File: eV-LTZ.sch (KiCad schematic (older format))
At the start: 28 parts, among them M1 SGP2, M2 SGP2, M3 SGP2, P1 CONN_01X04, P2 CONN_01X02, Q1 Q_NPN_EBC, U1 LT1013

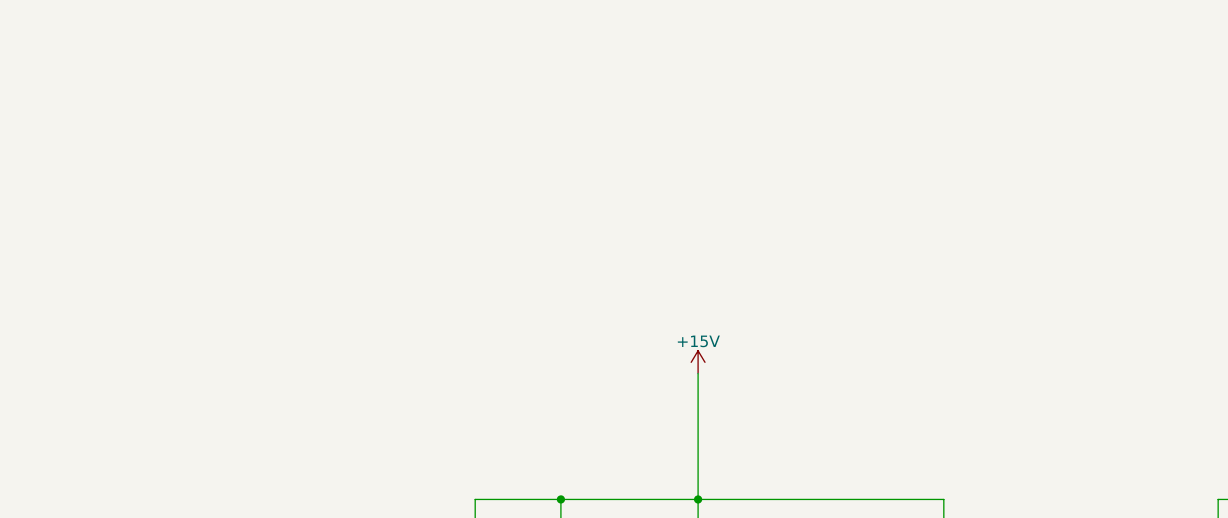
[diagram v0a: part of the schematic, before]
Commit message: TiN comments
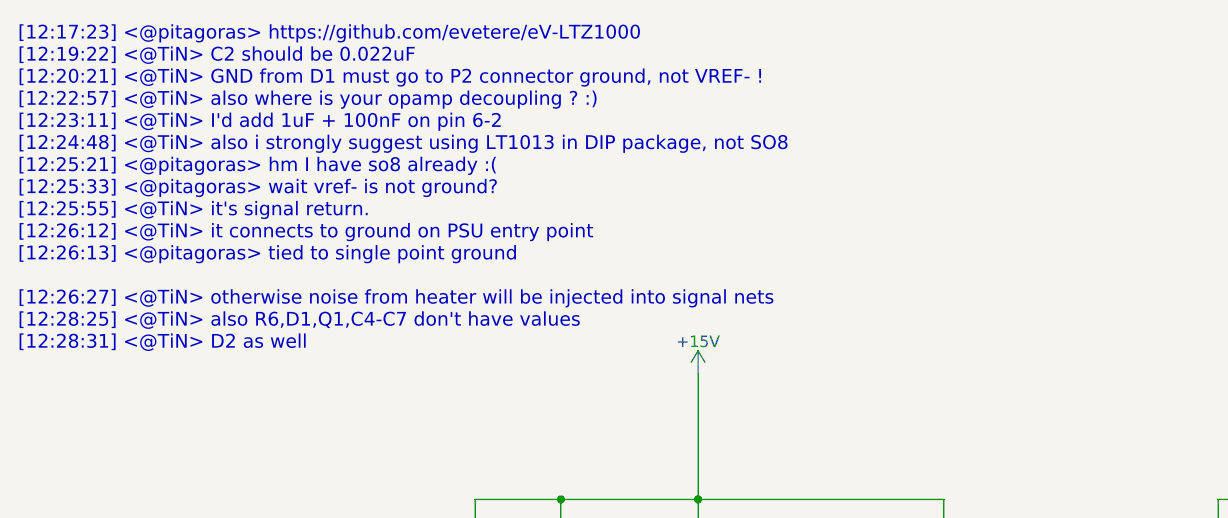
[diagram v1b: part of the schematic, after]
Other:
- note added: "[12:17:23] <@pitagoras> https://github.com/evetere/eV-LTZ1000\n[12:19:22] <@TiN> C2 should be 0.022uF\n[12:20:21] <@TiN> GND from D1 must go to P2 connector ground, not VREF- !\n[12:22:57] <@TiN> also where is your opamp decoupling ? :)\n[12:23:11] <@TiN> I'd add 1uF + 100nF on pin 6-2\n[12:24:48] <@TiN> also i strongly suggest using LT1013 in DIP package, not SO8\n[12:25:21] <@pitagoras> hm I ha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"
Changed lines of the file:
@@
 LIBS:valves
 LIBS:eV-LTZ1000
-LIBS:pi-LTZ-cache
+LIBS:eV-LTZ-cache
 EELAYER 25 0
 EELAYER END
@@
 Wire Wire Line
 	6300 3000 6300 2875
+Text Notes 1050 1900 0    60   ~ 0
+[12:17:23] <@pitagoras> https://github.com/evetere/eV-LTZ1000\n[12:19:22] <@TiN> C2 should be 0.022uF\n[12:20:21] <@TiN> GND from D1 must go to P2 connector ground, not VREF- !\n[12:22:57] <@TiN> also where is your opamp decoupling ? :)\n[12:23:11] <@TiN> I'd add 1uF + 100nF on pin 6-2\n[12:24:48] <@TiN> also i strongly suggest using LT1013 in DIP package, not SO8\n[12:25:21] <@pitagoras> hm I have so8 already :(\n[12:25:33] <@pitagoras> wait vref- is not ground?\n[12:25:55] <@TiN> it's signal return.\n[12:26:12] <@TiN> it connects to ground on PSU entry point\n[12:26:13] <@pitagoras> tied to single point ground \n\n[12:26:27] <@TiN> otherwise noise from heater will be injected into signal nets\n[12:28:25] <@TiN> also R6,D1,Q1,C4-C7 don't have values\n[12:28:31] <@TiN> D2 as well\n\n
 $EndSCHEMATC

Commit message: fix TiN comments
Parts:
- removed C5: C, symbol C
- added C? (x2): 1u, symbol CP
- C2: value 0.002uF -> 0.022uF
- C4, C6: value C -> 100n
- C7: value C -> 0.022uF
- D1, D2: value D -> 1N4148
- P1: value CONN_01X04 -> REF
- P2: value CONN_01X02 -> PWR
- Q1: value Q_NPN_EBC -> 2N3904
- R6: value R -> 1k
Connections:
- wire segments 82 -> 85
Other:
- note removed: "[12:17:23] <@pitagoras> https://github.com/evetere/eV-LTZ1000\n[12:19:22] <@TiN> C2 should be 0.022uF\n[12:20:21] <@TiN> GND from D1 must go to P2 connector ground, not VREF- !\n[12:22:57] <@TiN> also where is your opamp decoupling ? :)\n[12:23:11] <@TiN> I'd add 1uF + 100nF on pin 6-2\n[12:24:48] <@TiN> also i strongly suggest using LT1013 in DIP package, not SO8\n[12:25:21] <@pitagoras> hm I ha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"
- moved on the sheet: C1, C6, C7, M3, R7
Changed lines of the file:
@@
 LIBS:valves
 LIBS:eV-LTZ1000
-LIBS:eV-LTZ-cache
 EELAYER 25 0
 EELAYER END
@@
 P 4500 3250
 F 0 "R6" V 4580 3250 50  0000 C CNN
-F 1 "R" V 4500 3250 50  0000 C CNN
+F 1 "1k" V 4500 3250 50  0000 C CNN
 F 2 "" V 4430 3250 50  0001 C CNN
 F 3 "" H 4500 3250 50  0000 C CNN
@@
 P 4525 4925
 F 0 "D1" H 4525 5025 50  0000 C CNN
-F 1 "D" H 4525 4825 50  0000 C CNN
+F 1 "1N4148" H 4525 4825 50  0000 C CNN
 F 2 "" H 4525 4925 50  0001 C CNN
 F 3 "" H 4525 4925 50  0000 C CNN
@@
 L C C1
 U 1 1 591A85DA
-P 5450 3900
-F 0 "C1" H 5475 4000 50  0000 L CNN
-F 1 ".1uF" H 5475 3800 50  0000 L CNN
-F 2 "" H 5488 3750 50  0001 C CNN
-F 3 "" H 5450 3900 50  0000 C CNN
-	1    5450 3900
+P 5600 3900
+F 0 "C1" H 5625 4000 50  0000 L CNN
+F 1 ".1uF" H 5625 3800 50  0000 L CNN
+F 2 "" H 5638 3750 50  0001 C CNN
+F 3 "" H 5600 3900 50  0000 C CNN
+	1    5600 3900
 	1    0    0    -1
 $EndComp
@@
 L R R7
 U 1 1 591A8697
-P 5450 3550
-F 0 "R7" V 5530 3550 50  0000 C CNN
-F 1 "1M" V 5450 3550 50  0000 C CNN
-F 2 "" V 5380 3550 50  0001 C CNN
-F 3 "" H 5450 3550 50  0000 C CNN
-	1    5450 3550
+P 5600 3550
+F 0 "R7" V 5680 3550 50  0000 C CNN
+F 1 "1M" V 5600 3550 50  0000 C CNN
+F 2 "" V 5530 3550 50  0001 C CNN
+F 3 "" H 5600 3550 50  0000 C CNN
+	1    5600 3550
 	1    0    0    -1
 $EndComp
@@
 P 9400 2675
 F 0 "D2" H 9400 2775 50  0000 C CNN
-F 1 "D" H 9400 2575 50  0000 C CNN
+F 1 "1N4148" H 9400 2575 50  0000 C CNN
 F 2 "" H 9400 2675 50  0001 C CNN
 F 3 "" H 9400 2675 50  0000 C CNN
@@
 P 8300 4025
 F 0 "C2" H 8325 4125 50  0000 L CNN
-F 1 "0.002uF" H 8325 3925 50  0000 L CNN
+F 1 "0.022uF" H 8325 3925 50  0000 L CNN
 F 2 "" H 8338 3875 50  0001 C CNN
 F 3 "" H 8300 4025 50  0000 C CNN
@@
 L GND #PWR2
 U 1 1 591A9570
-P 5600 5150
-F 0 "#PWR2" H 5600 4900 50  0001 C CNN
-F 1 "GND" H 5600 5000 50  0000 C CNN
-F 2 "" H 5600 5150 50  0000 C CNN
-F 3 "" H 5600 5150 50  0000 C CNN
-	1    5600 5150
+P 3425 5450
+F 0 "#PWR2" H 3425 5200 50  0001 C CNN
+F 1 "GND" H 3425 5300 50  0000 C CNN
+F 2 "" H 3425 5450 50  0000 C CNN
+F 3 "" H 3425 5450 50  0000 C CNN
+	1    3425 5450
 	1    0    0    -1
 $EndComp
@@
 P 10150 3550
 F 0 "P1" H 10150 3800 50  0000 C CNN
-F 1 "CONN_01X04" V 10250 3550 50  0000 C CNN
+F 1 "REF" V 10250 3550 50  0000 C CNN
 F 2 "" H 10150 3550 50  0001 C CNN
 F 3 "" H 10150 3550 50  0000 C CNN
@@
 P 4125 3250
 F 0 "Q1" H 4325 3300 50  0000 L CNN
-F 1 "Q_NPN_EBC" H 4325 3200 50  0000 L CNN
+F 1 "2N3904" H 4325 3200 50  0000 L CNN
 F 2 "" H 4325 3350 50  0000 C CNN
 F 3 "" H 4125 3250 50  0000 C CNN
@@
 L SGP2 M3
 U 1 1 59BA1924
-P 9650 4100
-F 0 "M3" H 9425 4100 60  0000 C CNN
-F 1 "SGP2" H 9425 3875 60  0001 C CNN
-F 2 "" H 9175 4225 60  0001 C CNN
-F 3 "" H 9175 4225 60  0001 C CNN
-	1    9650 4100
-	1    0    0    -1
+P 3625 5225
+F 0 "M3" H 3400 5225 60  0000 C CNN
+F 1 "SGP2" H 3400 5000 60  0001 C CNN
+F 2 "" H 3150 5350 60  0001 C CNN
+F 3 "" H 3150 5350 60  0001 C CNN
+	1    3625 5225
+	-1   0    0    1
 $EndComp
 $Comp
@@
 Text Label 8725 3825 0    60   ~ 0
 SENSE-
-Text Label 9800 4100 0    60   ~ 0
+Text Label 9800 4000 0    60   ~ 0
 VREF-
 $Comp
@@
 P 2625 3275
 F 0 "P2" H 2625 3425 50  0000 C CNN
-F 1 "CONN_01X02" V 2725 3275 50  0000 C CNN
+F 1 "PWR" V 2725 3275 50  0000 C CNN
 F 2 "" H 2625 3275 50  0000 C CNN
 F 3 "" H 2625 3275 50  0000 C CNN
@@
 L C C7
 U 1 1 59BC10DD
-P 4825 2800
-F 0 "C7" H 4850 2900 50  0000 L CNN
-F 1 "C" H 4850 2700 50  0000 L CNN
-F 2 "" H 4863 2650 50  0000 C CNN
-F 3 "" H 4825 2800 50  0000 C CNN
-	1    4825 2800
+P 4825 3575
+F 0 "C7" H 4850 3675 50  0000 L CNN
+F 1 "0.022uF" H 4850 3475 50  0000 L CNN
+F 2 "" H 4863 3425 50  0000 C CNN
+F 3 "" H 4825 3575 50  0000 C CNN
+	1    4825 3575
 	0    1    1    0
-$EndComp
-$Comp
-L C C5
-U 1 1 59BC16B9
-P 3425 3750
-F 0 "C5" H 3450 3850 50  0000 L CNN
-F 1 "C" H 3450 3650 50  0000 L CNN
-F 2 "" H 3463 3600 50  0000 C CNN
-F 3 "" H 3425 3750 50  0000 C CNN
-	1    3425 3750
-	1    0    0    -1
 $EndComp
 $Comp
 L C C6
 U 1 1 59BC172F
-P 3650 3750
-F 0 "C6" H 3675 3850 50  0000 L CNN
-F 1 "C" H 3675 3650 50  0000 L CNN
-F 2 "" H 3688 3600 50  0000 C CNN
-F 3 "" H 3650 3750 50  0000 C CNN
-	1    3650 3750
-	1    0    0    -1
-$EndComp
-$Comp
-L C C4
-U 1 1 59BC1B82
-P 3200 3750
-F 0 "C4" H 3225 3850 50  0000 L CNN
-F 1 "C" H 3225 3650 50  0000 L CNN
-F 2 "" H 3238 3600 50  0000 C CNN
-F 3 "" H 3200 3750 50  0000 C CNN
-	1    3200 3750
+P 5400 3850
+F 0 "C6" H 5425 3950 50  0000 L CNN
+F 1 "100n" H 5425 3750 50  0000 L CNN
+F 2 "" H 5438 3700 50  0000 C CNN
+F 3 "" H 5400 3850 50  0000 C CNN
+	1    5400 3850
 	1    0    0    -1
 $EndComp
@@
 	4025 3450 4025 4125
 Wire Wire Line
-	5450 4050 5450 4100
+	5600 4050 5600 4100
 Wire Wire Line
 	4025 4100 5900 4100
@@
 	5300 3350 5775 3350
 Wire Wire Line
-	5450 3400 5450 3350
-Connection ~ 5450 3350
-Wire Wire Line
-	5450 3700 5450 3750
+	5600 3400 5600 3350
+Connection ~ 5600 3350
+Wire Wire Line
+	5600 3700 5600 3750
 Wire Wire Line
 	4375 4925 4025 4925
 Wire Wire Line
 	4025 4925 4025 4900
-Wire Wire Line
-	4675 4925 9425 4925
 Connection ~ 5100 4925
 Wire Wire Line
 	6800 3550 6800 3650
-Connection ~ 5450 4100
+Connection ~ 5600 4100
 Wire Wire Line
 	5725 2975 5725 4150
@@
 	5100 2450 5100 2950
 Wire Wire Line
-	3050 2450 5100 2450
+	3050 2450 5400 2450
 Connection ~ 4025 2450
 Wire Wire Line
-	5725 4750 9100 4750
-Wire Wire Line
-	5100 5225 5100 3550
+	5325 4750 9100 4750
 Connection ~ 6300 4750
 Connection ~ 7200 4750
@@
 	6800 3650 7800 3650
 Wire Wire Line
-	9425 4925 9425 4200
-Wire Wire Line
-	9425 4200 9550 4200
-Wire Wire Line
 	9100 4750 9100 4000
 Wire Wire Line
-	9100 4000 9550 4000
+	9100 4000 9800 4000
 Wire Wire Line
 	9600 3600 9950 3600
 Wire Wire Line
-	9650 4100 9800 4100
-Wire Wire Line
-	9800 4100 9800 3700
-Wire Wire Line
 	9800 3700 9950 3700
 Wire Wire Line
@@
 	9600 3825 9600 3600
 Wire Wire Line
-	5600 5150 5600 4925
-Connection ~ 5600 4925
+	3425 3900 3425 5450
+Connection ~ 3425 5225
 Wire Wire Line
 	2825 3225 3050 3225
@@
 	3050 3325 3050 5225
 Wire Wire Line
-	3050 5225 5100 5225
-Wire Wire Line
-	4975 2800 5325 2800
-Wire Wire Line
-	5325 2800 5325 3350
-Connection ~ 5325 3350
+	4975 3575 5300 3575
+Connection ~ 5300 3350
 Connection ~ 4675 3250
-Wire Wire Line
-	4675 3250 4675 2800
 Wire Wire Line
 	3425 2450 3425 3600
 Connection ~ 3425 2450
-Wire Wire Line
-	3200 3900 3650 3900
 Connection ~ 3425 3900
 Wire Wire Line
 	3200 3600 3200 3500
-Wire Wire Line
-	3200 3500 3650 3500
 Connection ~ 3425 3500
 Wire Wire Line
-	3650 3500 3650 3600
-Wire Wire Line
-	3425 3900 3425 5225
-Connection ~ 3425 5225
-Wire Wire Line
 	6300 3000 6300 2875
-Text Notes 1050 1900 0    60   ~ 0
-[12:17:23] <@pitagoras> https://github.com/evetere/eV-LTZ1000\n[12:19:22] <@TiN> C2 should be 0.022uF\n[12:20:21] <@TiN> GND from D1 must go to P2 connector ground, not VREF- !\n[12:22:57] <@TiN> also where is your opamp decoupling ? :)\n[12:23:11] <@TiN> I'd add 1uF + 100nF on pin 6-2\n[12:24:48] <@TiN> also i strongly suggest using LT1013 in DIP package, not SO8\n[12:25:21] <@pitagoras> hm I have so8 already :(\n[12:25:33] <@pitagoras> wait vref- is not ground?\n[12:25:55] <@TiN> it's signal return.\n[12:26:12] <@TiN> it connects to ground on PSU entry point\n[12:26:13] <@pitagoras> tied to single point ground \n\n[12:26:27] <@TiN> otherwise noise from heater will be injected into signal nets\n[12:28:25] <@TiN> also R6,D1,Q1,C4-C7 don't have values\n[12:28:31] <@TiN> D2 as well\n\n
+Wire Wire Line
+	5300 3575 5300 3350
+Wire Wire Line
+	4675 3575 4675 3250
+$Comp
+L CP C?
+U 1 1 59CD714F
+P 5200 3850
+F 0 "C?" H 5225 3950 50  0000 L CNN
+F 1 "1u" H 5225 3750 50  0000 L CNN
+F 2 "" H 5238 3700 50  0000 C CNN
+F 3 "" H 5200 3850 50  0000 C CNN
+	1    5200 3850
+	1    0    0    -1
+$EndComp
+Wire Wire Line
+	5100 4050 5400 4050
+Wire Wire Line
+	5400 4050 5400 4000
+Connection ~ 5100 4050
+Wire Wire Line
+	5200 4000 5200 4050
+Connection ~ 5200 4050
+Wire Wire Line
+	5200 3700 5400 3700
+Wire Wire Line
+	5400 3700 5400 2450
+Connection ~ 5100 2450
+$Comp
+L C C4
+U 1 1 59BC1B82
+P 3200 3750
+F 0 "C4" H 3225 3850 50  0000 L CNN
+F 1 "100n" H 3225 3650 50  0000 L CNN
+F 2 "" H 3238 3600 50  0000 C CNN
+F 3 "" H 3200 3750 50  0000 C CNN
+	1    3200 3750
+	1    0    0    -1
+$EndComp
+$Comp
+L CP C?
+U 1 1 59CD7798
+P 3425 3750
+F 0 "C?" H 3450 3850 50  0000 L CNN
+F 1 "1u" H 3450 3650 50  0000 L CNN
+F 2 "" H 3463 3600 50  0000 C CNN
+F 3 "" H 3425 3750 50  0000 C CNN
+	1    3425 3750
+	1    0    0    -1
+$EndComp
+Wire Wire Line
+	3200 3500 3425 3500
+Wire Wire Line
+	3200 3900 3425 3900
+Wire Wire Line
+	3050 5225 3625 5225
+Wire Wire Line
+	5100 4925 4675 4925
+Wire Wire Line
+	5100 5125 3725 5125
+Wire Wire Line
+	5325 5325 3725 5325
+Wire Wire Line
+	5325 4750 5325 5325
+Wire Wire Line
+	5100 3550 5100 5125
+Connection ~ 5725 4750
+Wire Wire Line
+	9800 4000 9800 3700
 $EndSCHEMATC

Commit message: guard ring
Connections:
- wire segments 85 -> 120
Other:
- note added: "guard ring"
- moved on the sheet: C1, C4, C6, C7, D1, M3, P2, Q1, R6, R7, U1A

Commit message: updates
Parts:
- removed C?: 1u, symbol CP
- removed M1, M2, M3: SGP2, symbol SGP2
- removed P1: REF, symbol CONN_01X04
- removed Q1: 2N3904, symbol Q_NPN_EBC
- removed R4.3: 0k, symbol R
- removed U1: LT1013, symbol LT1013
- added C10, C5: 1uF, Capacitors_THT:CP_Radial_Tantal_D5.0mm_P5.00mm, symbol CP
- added C9: .1uF, Capacitors_THT:C_Rect_L7.2mm_W2.5mm_P5.00mm_FKS2_FKP2_MKS2_MKP2, symbol C
- added D3, D6: 1N5819, Diodes_THT:D_DO-41_SOD81_P10.16mm_Horizontal, symbol D_Shockley
- added D4, D5, D7: D_TVS, Diodes_THT:D_DO-15_P10.16mm_Horizontal, symbol D_TVS
- added P1: VIN+, Connectors:1pin, symbol CONN_01X01
- added P3: VH-, Connectors:1pin, symbol CONN_01X01
- added P4: VH+, Connectors:1pin, symbol CONN_01X01
- added P5: SENSE-, Connectors:1pin, symbol CONN_01X01
- added P6: SENSE+, Connectors:1pin, symbol CONN_01X01
- added P7: VIN-, Connectors:1pin, symbol CONN_01X01
- added Q1: BD139, TO_SOT_Packages_THT:TO-126_Vertical, symbol BD139
- added R4: 100k, Resistors_THT:R_Axial_DIN0309_L9.0mm_D3.2mm_P12.70mm_Horizontal, symbol R
- added TH1: 10k, Varistors:RV_Disc_D7_W3.4_P5, symbol Thermistor_NTC
- added U1: LT1013N8, Housings_DIP:DIP-8_W7.62mm, symbol LT1013N8
- added W1: TEST_HEATER, Connectors:PINTST, symbol TEST_1P
- added W2: TEST_SENSE, Connectors:PINTST, symbol TEST_1P
- C1, C2, C7: footprint (none) -> Capacitors_THT:C_Rect_L7.2mm_W2.5mm_P5.00mm_FKS2_FKP2_MKS2_MKP2
- C3: value 0.1uF -> .1uF; footprint (none) -> Capacitors_THT:C_Rect_L7.2mm_W2.5mm_P5.00mm_FKS2_FKP2_MKS2_MKP2
- C4, C6: value 100n -> .1uF; footprint (none) -> Capacitors_THT:C_Rect_L7.2mm_W2.5mm_P5.00mm_FKS2_FKP2_MKS2_MKP2
- C8: renamed from C?; value 1u -> 1uF; footprint (none) -> Capacitors_THT:CP_Radial_Tantal_D5.0mm_P5.00mm
- D1, D2: footprint (none) -> Diodes_THT:D_A-405_P7.62mm_Horizontal
- P2: value PWR -> CONN_01X02; footprint (none) -> Connectors:bornier2
- R1, R2, R3, R4.1, R4.2, R5: footprint (none) -> Resistors_THT:R_Axial_DIN0614_L14.3mm_D5.7mm_P15.24mm_Horizontal
- R6, R7, R8, R9: footprint (none) -> Resistors_THT:R_Axial_DIN0309_L9.0mm_D3.2mm_P12.70mm_Horizontal
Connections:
- net labels added: HEAT, TSENSE, VH+, VH-, VIN+, VIN-
- net labels removed: +15V, VREF-
- wire segments 120 -> 97
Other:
- moved on the sheet: C1, C2, C3, C4, C6, C7, D1, D2, R1, R2, R3, R4.1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

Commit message: pcb
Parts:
- removed C8: 1uF, Capacitors_THT:CP_Radial_Tantal_D5.0mm_P5.00mm, symbol CP
- removed C9: .1uF, Capacitors_THT:C_Rect_L7.2mm_W2.5mm_P5.00mm_FKS2_FKP2_MKS2_MKP2, symbol C
- removed D4, D5, D7: D_TVS, Diodes_THT:D_DO-15_P10.16mm_Horizontal, symbol D_TVS
- C10, C5: value 1uF -> 47uF
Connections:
- wire segments 97 -> 89
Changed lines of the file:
@@
-$EndComp
-$Comp
-L CP C8
-U 1 1 59CD714F
-P 5175 2975
-F 0 "C8" H 5200 3075 50  0000 L CNN
-F 1 "1uF" H 5200 2875 50  0000 L CNN
-F 2 "Capacitors_THT:CP_Radial_Tantal_D5.0mm_P5.00mm" H 5213 2825 50  0001 C CNN
-F 3 "" H 5175 2975 50  0000 C CNN
-	1    5175 2975
-	1    0    0    -1
 $EndComp
 $Comp
@@
 	1    6300 925
 	1    0    0    -1
-$EndComp
-$Comp
-L D_TVS D5
-U 1 1 59EE5901
-P 1650 3125
-F 0 "D5" H 1650 3225 50  0000 C CNN
-F 1 "D_TVS" H 1650 3025 50  0000 C CNN
-F 2 "Diodes_THT:D_DO-15_P10.16mm_Horizontal" H 1650 3125 50  0001 C CNN
-F 3 "" H 1650 3125 50  0000 C CNN
-	1    1650 3125
-	0    1    1    0
 $EndComp
 $Comp
@@
 $EndComp
 $Comp
-L C C9
-U 1 1 59FDB55A
-P 3050 3275
-F 0 "C9" H 3075 3375 50  0000 L CNN
-F 1 ".1uF" H 3075 3175 50  0000 L CNN
-F 2 "Capacitors_THT:C_Rect_L7.2mm_W2.5mm_P5.00mm_FKS2_FKP2_MKS2_MKP2" H 3088 3125 50  0001 C CNN
-F 3 "" H 3050 3275 50  0000 C CNN
-	1    3050 3275
-	1    0    0    -1
-$EndComp
-$Comp
 L D_Shockley D6
 U 1 1 59FDD6C1
@@
 	1    0    0    -1
 $EndComp
-$Comp
-L D_TVS D4
-U 1 1 59FDF05E
-P 1900 3125
-F 0 "D4" H 1900 3225 50  0000 C CNN
-F 1 "D_TVS" H 1900 3025 50  0000 C CNN
-F 2 "Diodes_THT:D_DO-15_P10.16mm_Horizontal" H 1900 3125 50  0001 C CNN
-F 3 "" H 1900 3125 50  0000 C CNN
-	1    1900 3125
-	0    1    1    0
-$EndComp
 Wire Wire Line
 	6325 2475 6750 2475
@@
 Connection ~ 5075 3175
 Wire Wire Line
-	5175 3125 5175 3175
-Connection ~ 5175 3175
-Wire Wire Line
-	5375 2825 5175 2825
-Wire Wire Line
 	5375 1475 5375 2825
 Connection ~ 5075 1475
@@
 	1900 1675 1900 2975
 Connection ~ 1900 1675
-$Comp
-L D_TVS D7
-U 1 1 59FE08AF
-P 10100 2525
-F 0 "D7" H 10100 2625 50  0000 C CNN
-F 1 "D_TVS" H 10100 2425 50  0000 C CNN
-F 2 "Diodes_THT:D_DO-15_P10.16mm_Horizontal" H 10100 2525 50  0001 C CNN
-F 3 "" H 10100 2525 50  0000 C CNN
-	1    10100 2525
-	0    1    1    0
-$EndComp
-Wire Wire Line
-	10100 1925 10100 2375
 Connection ~ 10100 1925
-Wire Wire Line
-	10100 2675 10100 3075
 Connection ~ 10100 3075
 $Comp
@@
 	4000 4100 4000 4025
 Connection ~ 3375 1675
-Wire Wire Line
-	3050 1475 3050 3125
 Connection ~ 3050 1475
 Connection ~ 5075 3875
@@
 L CP C5
 U 1 1 59FE960F
-P 2775 3275
-F 0 "C5" H 2800 3375 50  0000 L CNN
-F 1 "1uF" H 2800 3175 50  0000 L CNN
-F 2 "Capacitors_THT:CP_Radial_Tantal_D5.0mm_P5.00mm" H 2813 3125 50  0001 C CNN
-F 3 "" H 2775 3275 50  0000 C CNN
-	1    2775 3275
-	1    0    0    -1
-$EndComp
-Wire Wire Line
-	2775 3125 2775 2650
-Wire Wire Line
-	2775 2650 3050 2650
-Connection ~ 3050 2650
-Wire Wire Line
-	2775 3425 2775 3675
-Wire Wire Line
-	2775 3675 3050 3675
-Connection ~ 3050 3675
+P 3050 3275
+F 0 "C5" H 3075 3375 50  0000 L CNN
+F 1 "47uF" H 3075 3175 50  0000 L CNN
+F 2 "Capacitors_THT:CP_Radial_Tantal_D5.0mm_P5.00mm" H 3088 3125 50  0001 C CNN
+F 3 "" H 3050 3275 50  0000 C CNN
+	1    3050 3275
+	1    0    0    -1
+$EndComp
 $Comp
 L R R4
@@
 P 3650 3375
 F 0 "C10" H 3675 3475 50  0000 L CNN
-F 1 "1uF" H 3675 3275 50  0000 L CNN
+F 1 "47uF" H 3675 3275 50  0000 L CNN
 F 2 "Capacitors_THT:CP_Radial_Tantal_D5.0mm_P5.00mm" H 3688 3225 50  0001 C CNN
 F 3 "" H 3650 3375 50  0000 C CNN
@@
 	-1   0    0    1
 $EndComp
+Wire Wire Line
+	3050 1475 3050 3125
 $EndSCHEMATC

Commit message: change footprint
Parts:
- removed R4.2: 25k, Resistors_THT:R_Axial_DIN0614_L14.3mm_D5.7mm_P15.24mm_Horizontal, symbol R
- R1, R2, R3, R5: footprint Resistors_THT:R_Axial_DIN0614_L14.3mm_D5.7mm_P15.24mm_Horizontal -> Resistors_THT:R_Axial_DIN0617_L17.0mm_D6.0mm_P20.32mm_Horizontal
- R4.1: value 25k -> 12k; footprint Resistors_THT:R_Axial_DIN0614_L14.3mm_D5.7mm_P15.24mm_Horizontal -> Resistors_THT:R_Axial_DIN0617_L17.0mm_D6.0mm_P20.32mm_Horizontal
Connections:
- wire segments 89 -> 87
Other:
- moved on the sheet: R4.1
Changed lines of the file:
@@
 LIBS:sensors
 LIBS:lp2951
-LIBS:eV-LTZ-cache
 EELAYER 25 0
 EELAYER END
@@
 F 0 "R3" V 7130 1850 50  0000 C CNN
 F 1 "70k" V 7050 1850 50  0000 C CNN
-F 2 "Resistors_THT:R_Axial_DIN0614_L14.3mm_D5.7mm_P15.24mm_Horizontal" V 6980 1850 50  0001 C CNN
+F 2 "Resistors_THT:R_Axial_DIN0617_L17.0mm_D6.0mm_P20.32mm_Horizontal" V 6980 1850 50  0001 C CNN
 F 3 "" H 7050 1850 50  0000 C CNN
 	1    7050 1850
-	1    0    0    -1
-$EndComp
-$Comp
-L R R4.2
-U 1 1 591A7C6A
-P 6650 1850
-F 0 "R4.2" V 6730 1850 50  0000 C CNN
-F 1 "25k" V 6650 1850 50  0000 C CNN
-F 2 "Resistors_THT:R_Axial_DIN0614_L14.3mm_D5.7mm_P15.24mm_Horizontal" V 6580 1850 50  0001 C CNN
-F 3 "" H 6650 1850 50  0000 C CNN
-	1    6650 1850
 	1    0    0    -1
 $EndComp
@@
 F 0 "R5" V 6630 2875 50  0000 C CNN
 F 1 "1k" V 6550 2875 50  0000 C CNN
-F 2 "Resistors_THT:R_Axial_DIN0614_L14.3mm_D5.7mm_P15.24mm_Horizontal" V 6480 2875 50  0001 C CNN
+F 2 "Resistors_THT:R_Axial_DIN0617_L17.0mm_D6.0mm_P20.32mm_Horizontal" V 6480 2875 50  0001 C CNN
 F 3 "" H 6550 2875 50  0000 C CNN
 	1    6550 2875
@@
 F 0 "R1" V 7530 3450 50  0000 C CNN
 F 1 "120" V 7450 3450 50  0000 C CNN
-F 2 "Resistors_THT:R_Axial_DIN0614_L14.3mm_D5.7mm_P15.24mm_Horizontal" V 7380 3450 50  0001 C CNN
+F 2 "Resistors_THT:R_Axial_DIN0617_L17.0mm_D6.0mm_P20.32mm_Horizontal" V 7380 3450 50  0001 C CNN
 F 3 "" H 7450 3450 50  0000 C CNN
 	1    7450 3450
@@
 F 0 "R2" V 8130 1775 50  0000 C CNN
 F 1 "70k" V 8050 1775 50  0000 C CNN
-F 2 "Resistors_THT:R_Axial_DIN0614_L14.3mm_D5.7mm_P15.24mm_Horizontal" V 7980 1775 50  0001 C CNN
+F 2 "Resistors_THT:R_Axial_DIN0617_L17.0mm_D6.0mm_P20.32mm_Horizontal" V 7980 1775 50  0001 C CNN
 F 3 "" H 8050 1775 50  0000 C CNN
 	1    8050 1775
@@
 L R R4.1
 U 1 1 59BA12BD
-P 6450 1850
-F 0 "R4.1" V 6530 1850 50  0000 C CNN
-F 1 "25k" V 6450 1850 50  0000 C CNN
-F 2 "Resistors_THT:R_Axial_DIN0614_L14.3mm_D5.7mm_P15.24mm_Horizontal" V 6380 1850 50  0001 C CNN
-F 3 "" H 6450 1850 50  0000 C CNN
-	1    6450 1850
+P 6550 1850
+F 0 "R4.1" V 6630 1850 50  0000 C CNN
+F 1 "12k" V 6550 1850 50  0000 C CNN
+F 2 "Resistors_THT:R_Axial_DIN0617_L17.0mm_D6.0mm_P20.32mm_Horizontal" V 6480 1850 50  0001 C CNN
+F 3 "" H 6550 1850 50  0000 C CNN
+	1    6550 1850
 	1    0    0    -1
 $EndComp
@@
 	7550 1925 10450 1925
 Wire Wire Line
-	6450 1700 6650 1700
-Wire Wire Line
-	6450 2000 6650 2000
-Connection ~ 6550 1700
-Connection ~ 6550 2000
-Wire Wire Line
 	7050 2925 8050 2925
